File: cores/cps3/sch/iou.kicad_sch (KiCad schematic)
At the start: 39 parts, among them CN1 Conn_01x34_Male, SW1 SW_MEC_5G

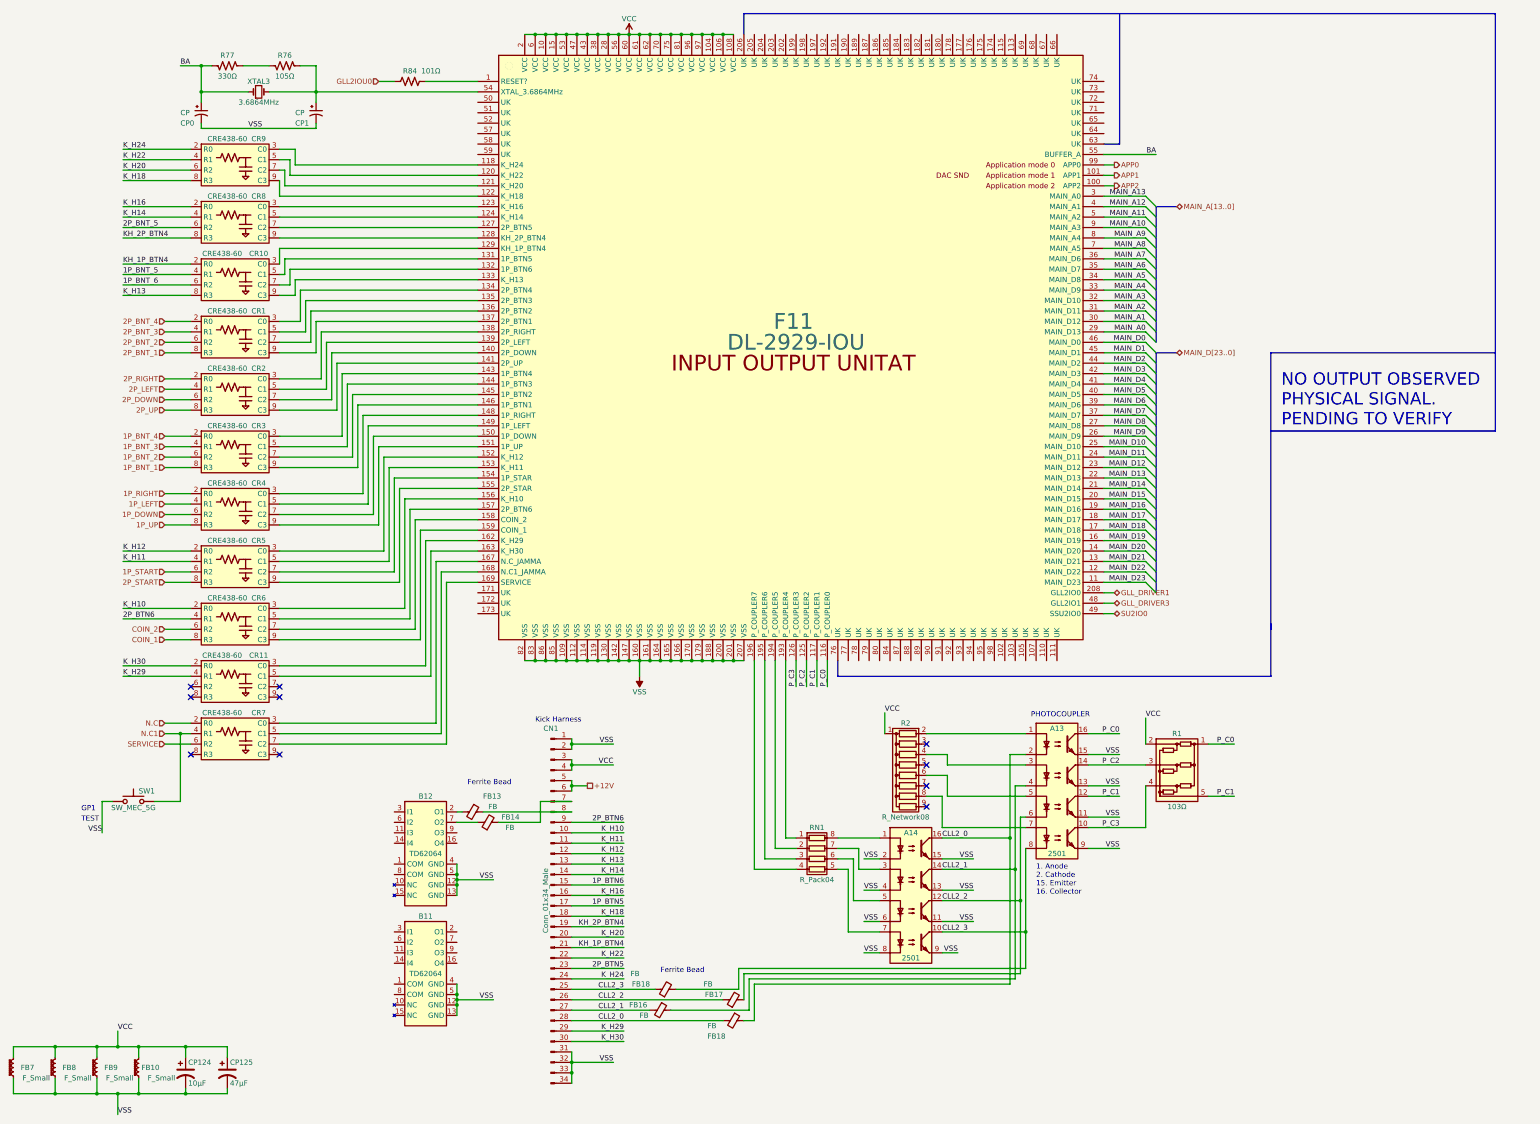
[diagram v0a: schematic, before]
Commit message: wip_iou_wd
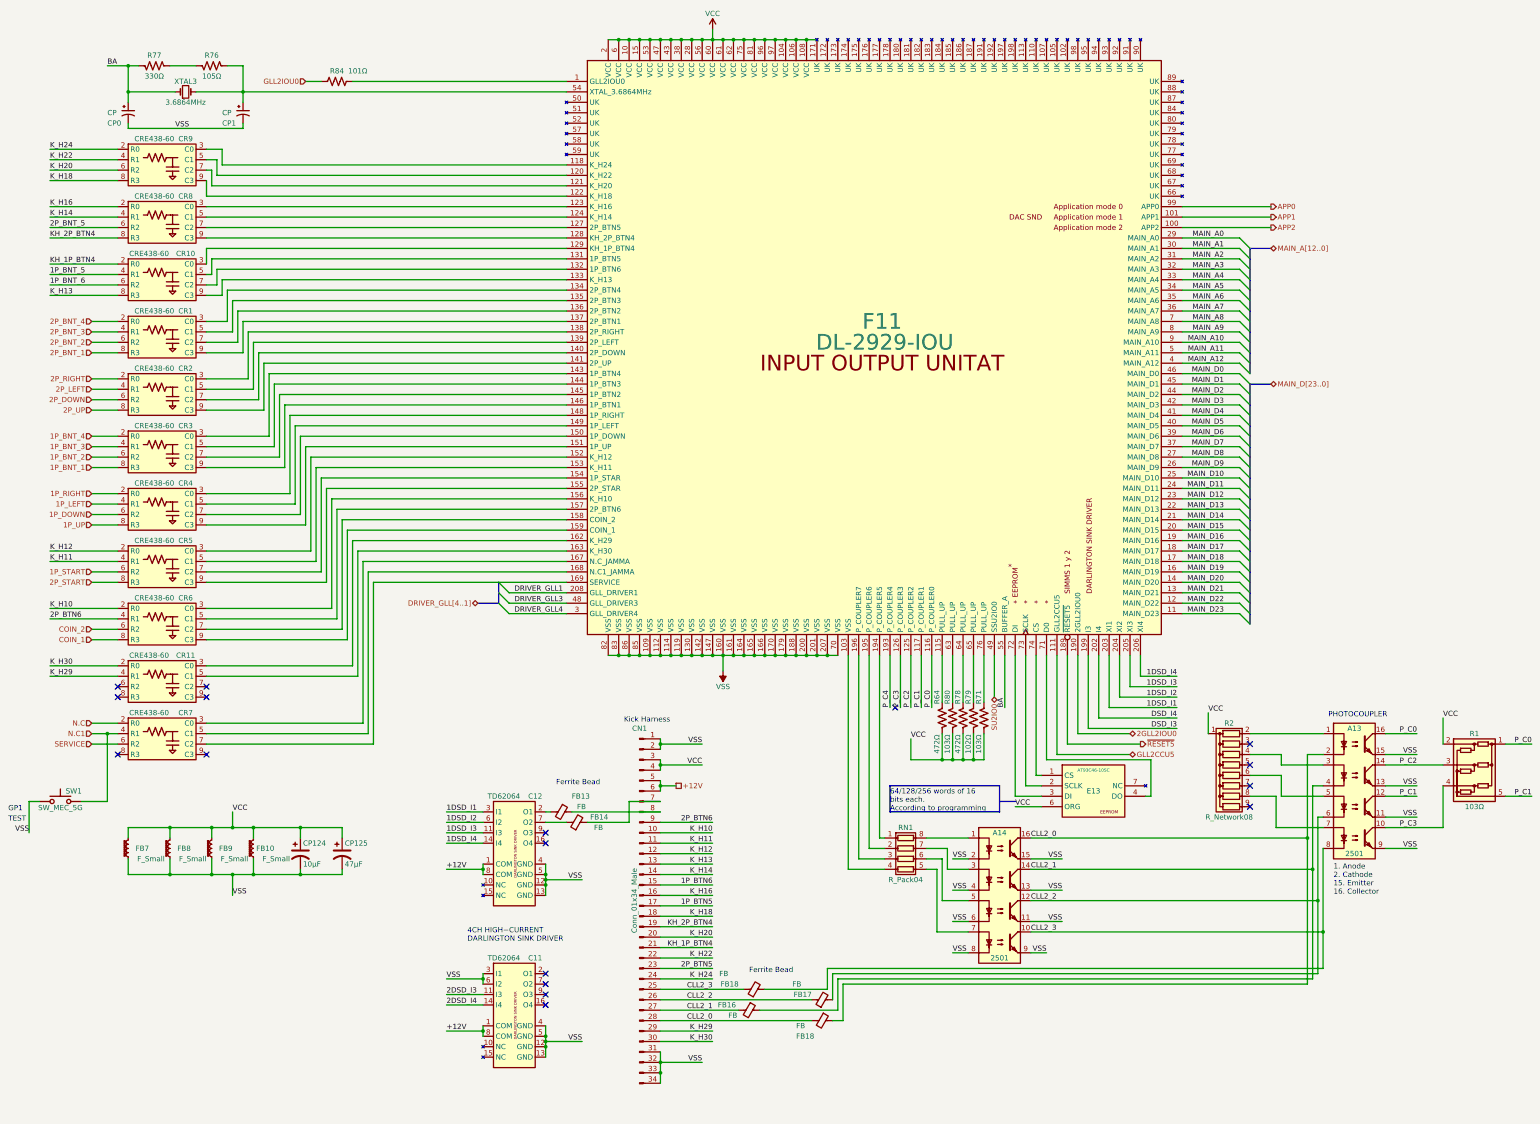
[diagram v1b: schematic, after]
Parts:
- removed B11: TD62064, symbol toshiba:TD62064
- added C11: TD62064, symbol toshiba:TD62064
- added E13: AT93C46-10SC, symbol arcade:AT93C46-10SC
- added R64, R78: 472Ω, symbol Device:R_US
- added R71, R80: 103Ω, symbol Device:R_US
- added R79: 102Ω, symbol Device:R_US
- renumbered B12 to C12
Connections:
- net +12V: now also C12.1 (COM), C12.8 (COM), C11.1 (COM), C11.8 (COM)
- net VCC: now also F11.171 (UK), E13.6 (ORG), E13.8 (VCC), R64.2, R71.2, R78.2, R79.2, R80.2; no longer F11.70 (VCC)
- net VSS: now also F11.70 (VSS), C11.12 (GND), C11.13 (GND), C11.3 (I1), C11.4 (GND), C11.5 (GND), C11.6 (I2), E13.5 (VSS)
- net at RN1.1 (R1.1): now also F11.194 (P_COUPLER5); no longer F11.193 (P_COUPLER4)
- net at RN1.2 (R2.1): now also F11.195 (P_COUPLER6); no longer F11.194 (P_COUPLER5)
- net at RN1.3 (R3.1): now also F11.196 (P_COUPLER7); no longer F11.195 (P_COUPLER6)
- net at RN1.4 (R4.1): now also F11.103 (VSS); no longer F11.196 (P_COUPLER7)
- net 1DSD_I3: now reaches C12.11 (I3)
- net 1DSD_I3: now also F11.205 (XI3)
- net 1DSD_I4: now reaches C12.14 (I4)
- net 1DSD_I4: now also F11.206 (XI4)
- net 1DSD_I1: now reaches C12.3 (I1)
- net 1DSD_I1: now also F11.203 (XI1)
- net 1DSD_I2: now reaches C12.6 (I2)
- net 1DSD_I2: now also F11.204 (XI2)
- net GLL2CCU5: now reaches F11.111 (GLL2CCU5)
- net at F11.115 (PULL_UP): now also R64.1
- net ~{RESET5}: now reaches F11.189 (~{RESET5})
- net 2GLL2IOU0: now reaches F11.190 (2GLL2IOU0)
- net DSD_I3: now reaches F11.199 (I3)
- net DSD_I4: now reaches F11.202 (I4)
- net at F11.63 (PULL_UP): now also R80.1
- net at F11.64 (PULL_UP): now also R78.1
- net at F11.65 (PULL_UP): now also R79.1
- net at F11.71 (D0): now also E13.4 (DO)
- net at F11.72 (DI): now also E13.3 (DI)
- net at F11.73 (SCLK): now also E13.2 (SCLK)
- net at F11.74 (CS): now also E13.1 (CS)
- net at F11.76 (PULL_UP): now also R71.1
- net GLL_DRIVER1 renamed DRIVER_GLL1
- net GLL_DRIVER3 renamed DRIVER_GLL3
- net MAIN_A13 renamed DRIVER_GLL4
- new net 2DSD_I3: C11.11 (I3)
- new net 2DSD_I4: C11.14 (I4)
- new net P_C4: F11.193 (P_COUPLER4)
- no-connect marks 10 -> 17
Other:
- note added: "4CH HIGH−CURRENT DARLINGTON SINK DRIVER"
- note added: "64/128/256 words of 16 bits each. According to programming"
- note removed: "NO OUTPUT OBSERVED PHYSICAL SIGNAL. PENDING TO VERIFY"
- moved on the sheet: A13, A14, CN1, CP0, CP1, CP124, CP125, CR1, CR10, CR11, CR2, CR3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
